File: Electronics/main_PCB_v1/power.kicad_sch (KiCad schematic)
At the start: 46 parts, among them J301 Conn_01x02, J305 Conn_01x02, J306 Conn_01x02, J307 Conn_01x02, J308 Conn_01x02, J309 Conn_01x02, J310 Conn_01x02, Q302 DMP3028LFDE, T301 NVMFS4C05NT1G, T302 NVMFS4C05NT1G, U301 LMR43620MB5RPER, U302 LMR43620MB5RPER, U303 LMR43620MB5RPER

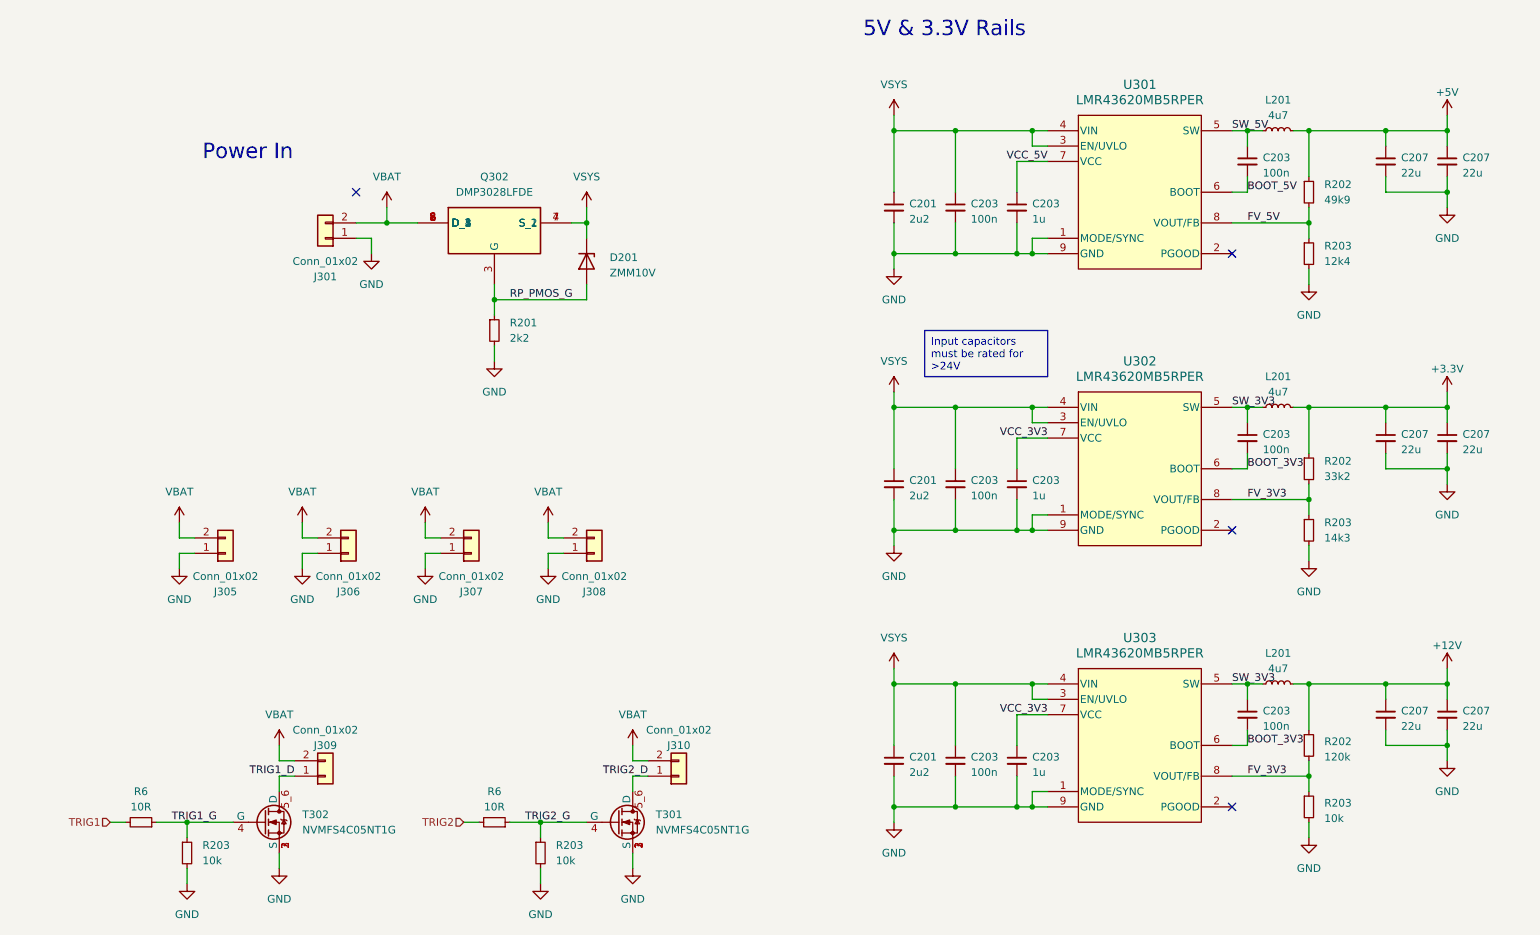
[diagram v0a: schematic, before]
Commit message: PCB Finished
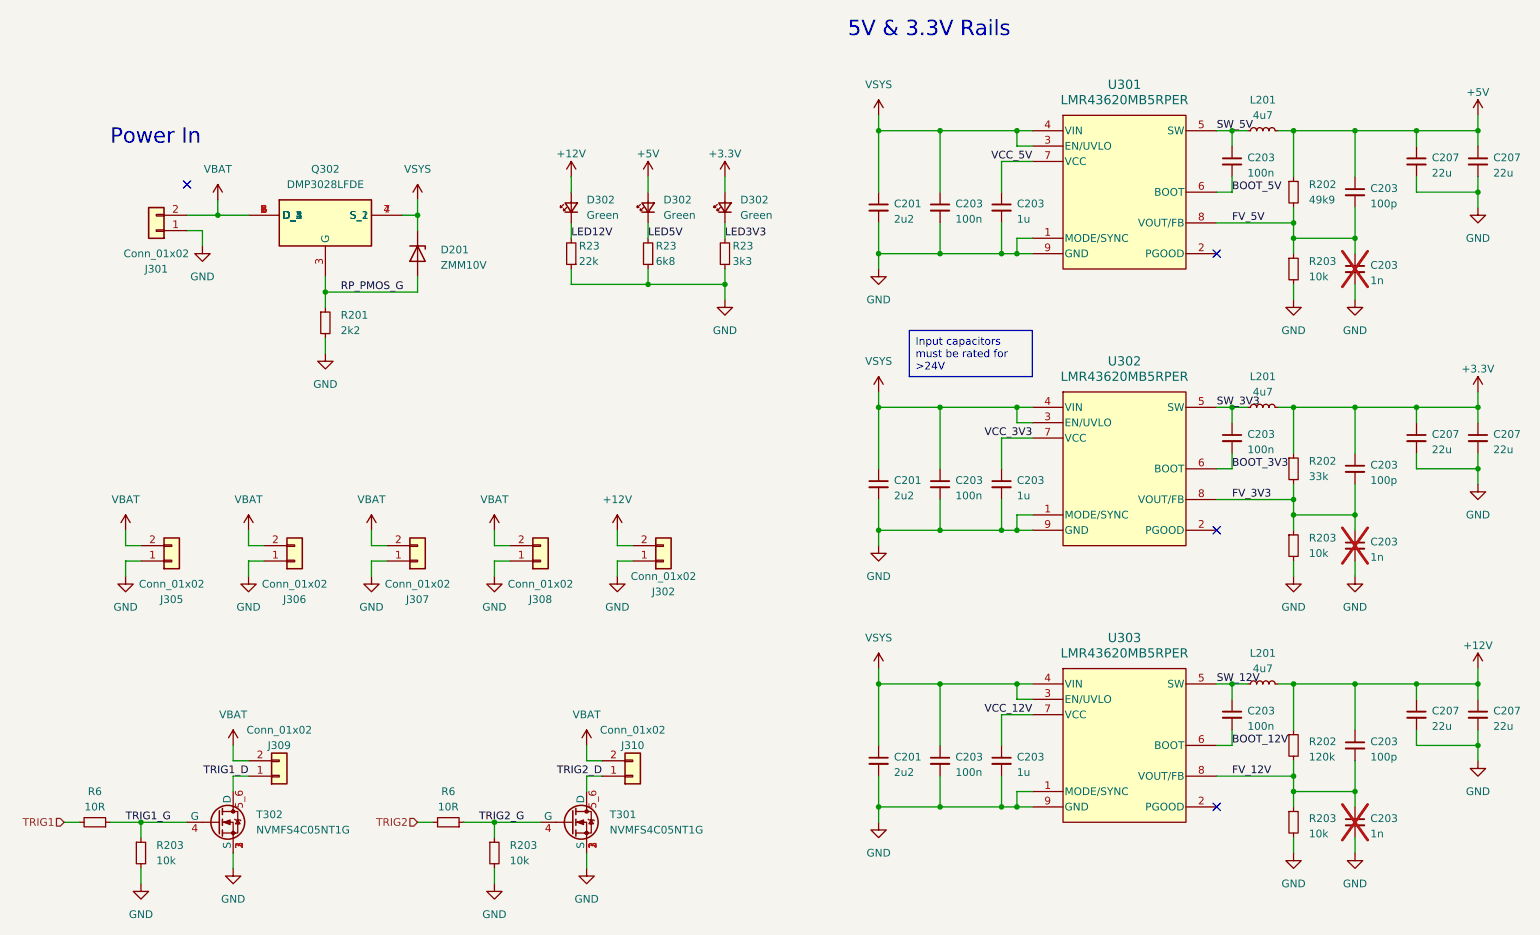
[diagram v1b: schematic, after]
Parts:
- added C203 (x3): 1n, Capacitor_SMD:C_0402_1005Metric, symbol Device:C_Small
- added C203 (x3): 100p, Capacitor_SMD:C_0402_1005Metric, symbol Device:C_Small
- added D302 (x3): Green, LED_SMD:LED_0603_1608Metric, symbol Device:LED_Small
- added J302: Conn_01x02, Connector_AMASS:AMASS_XT30U-F_1x02_P5.0mm_Vertical, symbol Connector_Generic:Conn_01x02
- added R23: 22k, Resistor_SMD:R_0402_1005Metric, symbol Device:R_Small
- added R23: 3k3, Resistor_SMD:R_0402_1005Metric, symbol Device:R_Small
- added R23: 6k8, Resistor_SMD:R_0402_1005Metric, symbol Device:R_Small
- R202: value 33k2 -> 33k
- R203: value 12k4 -> 10k
- R203: value 14k3 -> 10k
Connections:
- net +12V: now also C203.1, D302.2 (A), J302.2 (Pin_2)
- net +3.3V: now also C203.1, D302.2 (A)
- net +5V: now also C203.1, D302.2 (A)
- net BOOT_3V3: no longer C203.2, U303.6 (BOOT)
- net FV_3V3: now also C203.1, C203.2; no longer R202.2, R203.1, U303.8 (VOUT/FB)
- net FV_5V: now also C203.1, C203.2
- net GND: now also C203.2, C203.2, C203.2, J302.1 (Pin_1), R23.1, R23.1, R23.1
- net SW_3V3: no longer C203.1, L201.1, U303.5 (SW)
- net VCC_3V3: no longer C203.1, U303.7 (VCC)
- new net BOOT_12V: C203.2, U303.6 (BOOT)
- new net FV_12V: C203.1, C203.2, R202.2, R203.1, U303.8 (VOUT/FB)
- new net LED12V: D302.1 (K), R23.2
- new net LED3V3: D302.1 (K), R23.2
- new net LED5V: D302.1 (K), R23.2
- new net SW_12V: C203.1, L201.1, U303.5 (SW)
- new net VCC_12V: C203.1, U303.7 (VCC)
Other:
- moved on the sheet: C201, C203, C207, D201, J301, J305, J306, J307, J308, J309, J310, L201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
